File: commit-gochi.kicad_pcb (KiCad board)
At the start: 2 copper layers, 26.7 x 39.2 mm, 12 parts, among them J1 USB_C_Receptacle_USB2.0_16P, J2 Conn_01x04_Socket, Q1 Q_NPN_BCE, SW1 SW_Push, U1 ESP32-C3_SUPERMINI_TH

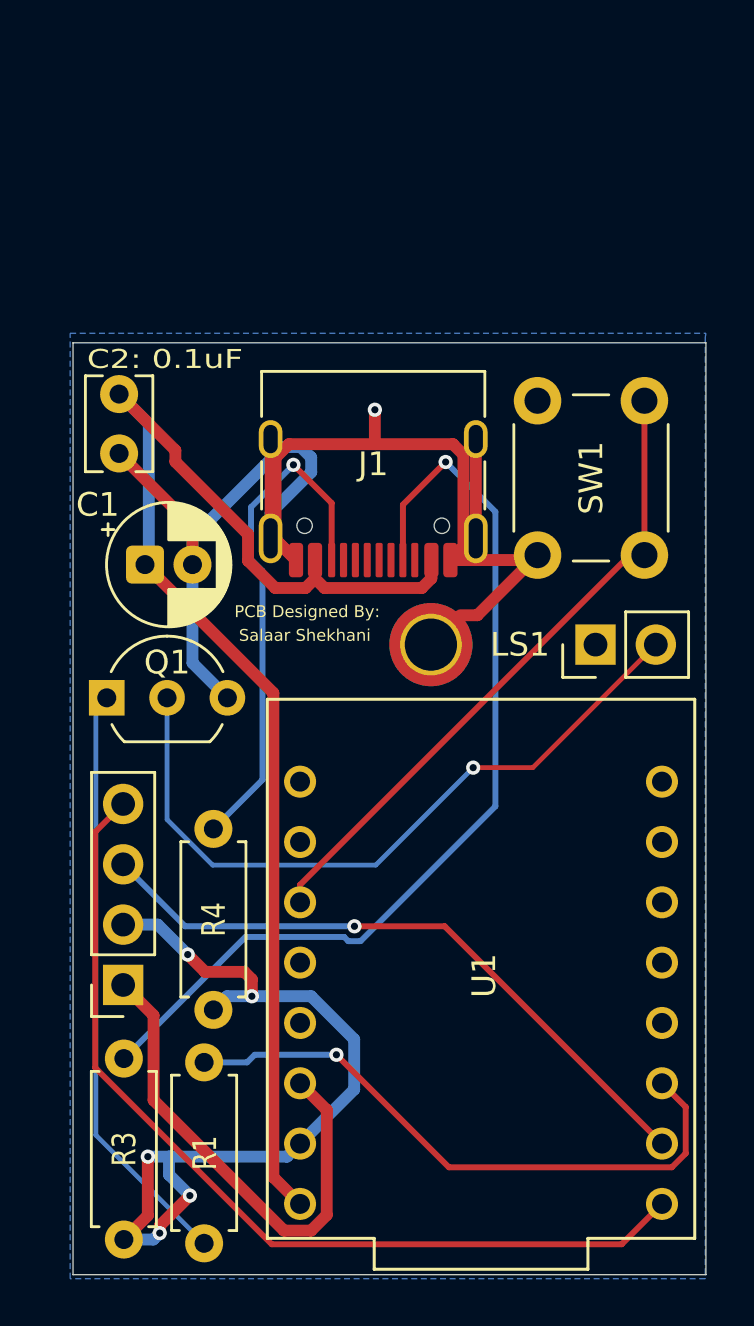
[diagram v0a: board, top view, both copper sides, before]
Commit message: Add files via upload
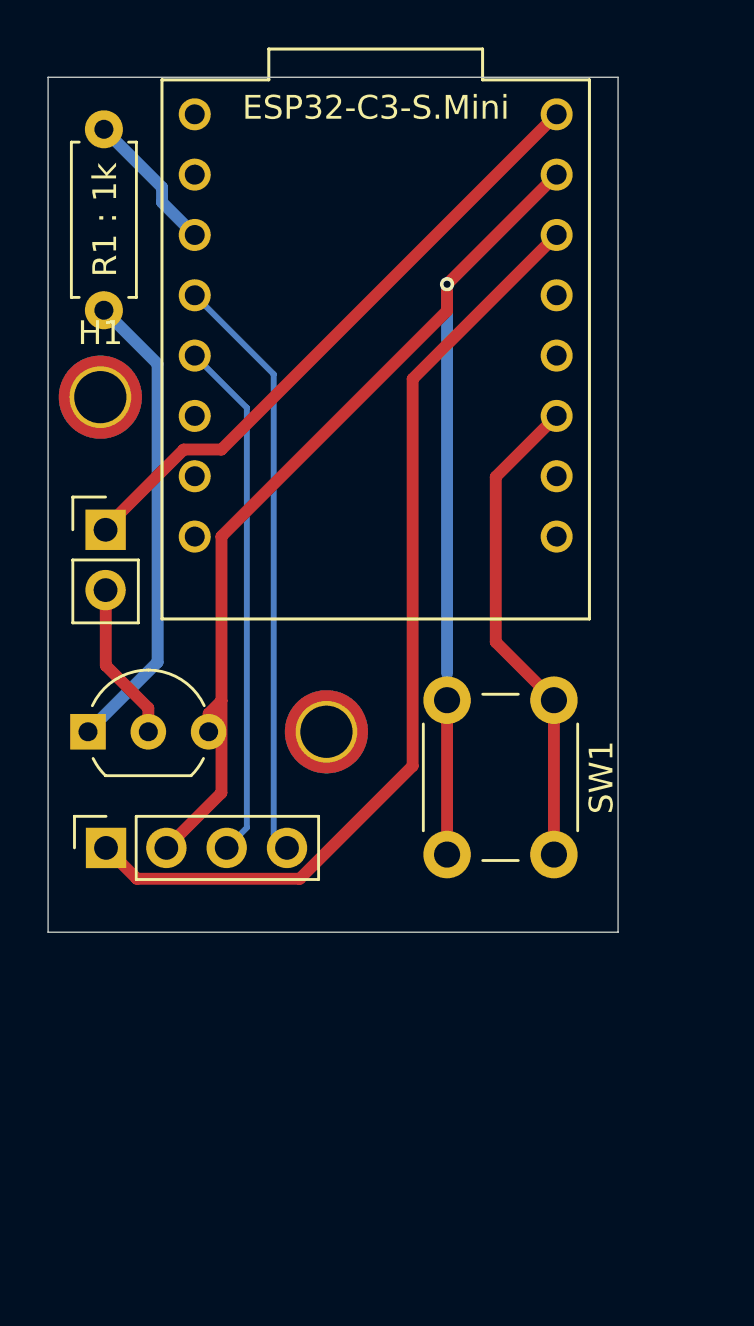
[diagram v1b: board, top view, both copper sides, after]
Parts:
- removed C1: 10uF, Capacitor_THT:CP_Radial_D5.0mm_P2.00mm
- removed C2: 0.1uF: 0.1uF, Capacitor_THT:C_Disc_D3.8mm_W2.6mm_P2.50mm
- removed J1: USB_C_Receptacle_USB2.0_16P, Connector_USB:USB_C_Receptacle_HRO_TYPE-C-31-M-12
- removed LS1: Speaker, Connector_PinHeader_2.54mm:PinHeader_1x02_P2.54mm_Vertical
- removed R1: 1k, Resistor_THT:R_Axial_DIN0207_L6.3mm_D2.5mm_P7.62mm_Horizontal
- removed R3, R4: 5.1k, Resistor_THT:R_Axial_DIN0207_L6.3mm_D2.5mm_P7.62mm_Horizontal
- removed Salaar Shekhani: MountingHole, MountingHole:MountingHole_2.2mm_M2_ISO7380_Pad_TopBottom
- removed U1: ESP32-C3_SUPERMINI_TH, c3:MODULE_ESP32-C3_SUPERMINI_TH
- added ESP32-C3-S.Mini: ESP32-C3_SUPERMINI_TH, c3:MODULE_ESP32-C3_SUPERMINI_TH, F.Cu at (86.8, 35.8)
- added H1: MountingHole, MountingHole:MountingHole_2.2mm_M2_ISO7380_Pad_TopBottom, F.Cu at (84.7, 51.9)
- added H1: MountingHole, MountingHole:MountingHole_2.2mm_M2_ISO7380_Pad_TopBottom, F.Cu at (75.2, 37.8)
- added R1 : 1k: 1k, Resistor_THT:R_Axial_DIN0207_L6.3mm_D2.5mm_P7.62mm_Horizontal, F.Cu at (75.3, 26.5)
- added Speaker: Speaker, Connector_PinHeader_2.54mm:PinHeader_1x02_P2.54mm_Vertical, F.Cu at (75.4, 43.4)
- moved SW1 13.2 mm to (94.3, 50.5)
- moved J2 5.81 mm to (75.4, 56.8), turned to 90 degrees
- moved Q1 1.63 mm to (74.7, 51.9)
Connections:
- net GND renamed Net-(J2-GND)
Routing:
- net Net-(C1-Pad1): track 57.4 -> 0.00 mm
- net Net-(J1-CC1): track 40.4 -> 0.00 mm, vias 1 -> 0
- net Net-(J2-GND): track 98.3 -> 59.6 mm, vias 6 -> 1
- net Net-(LS1-Pad1): track 0.00 -> 26.3 mm
- net Net-(Q1-C): track 30.3 -> 6.71 mm, vias 1 -> 0
- net Net-(J1-CC2): track 21.8 -> 0.00 mm, vias 1 -> 0
- net /SPEAKER_PWM: track 26.0 -> 6.03 mm, vias 1 -> 0
- net Net-(J2-VCC): track 21.2 -> 40.3 mm
- net /OLED_SDA: track 39.2 -> 24.9 mm
- net /BUTTON_IN: track 27.5 -> 20.5 mm
- net /OLED_SCL: track 27.6 -> 22.0 mm, vias 1 -> 0
- net Net-(Q1-B): track 25.0 -> 19.9 mm
- removed copper zone on B.Cu, net Net-(J2-GND)
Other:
- board size 26.7 x 39.2 mm -> 24 x 36 mm
- board text added: "Salaar Shekhani"
